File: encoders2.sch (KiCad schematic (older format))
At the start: 29 parts, among them U7 74HCT595, U9 74HC165

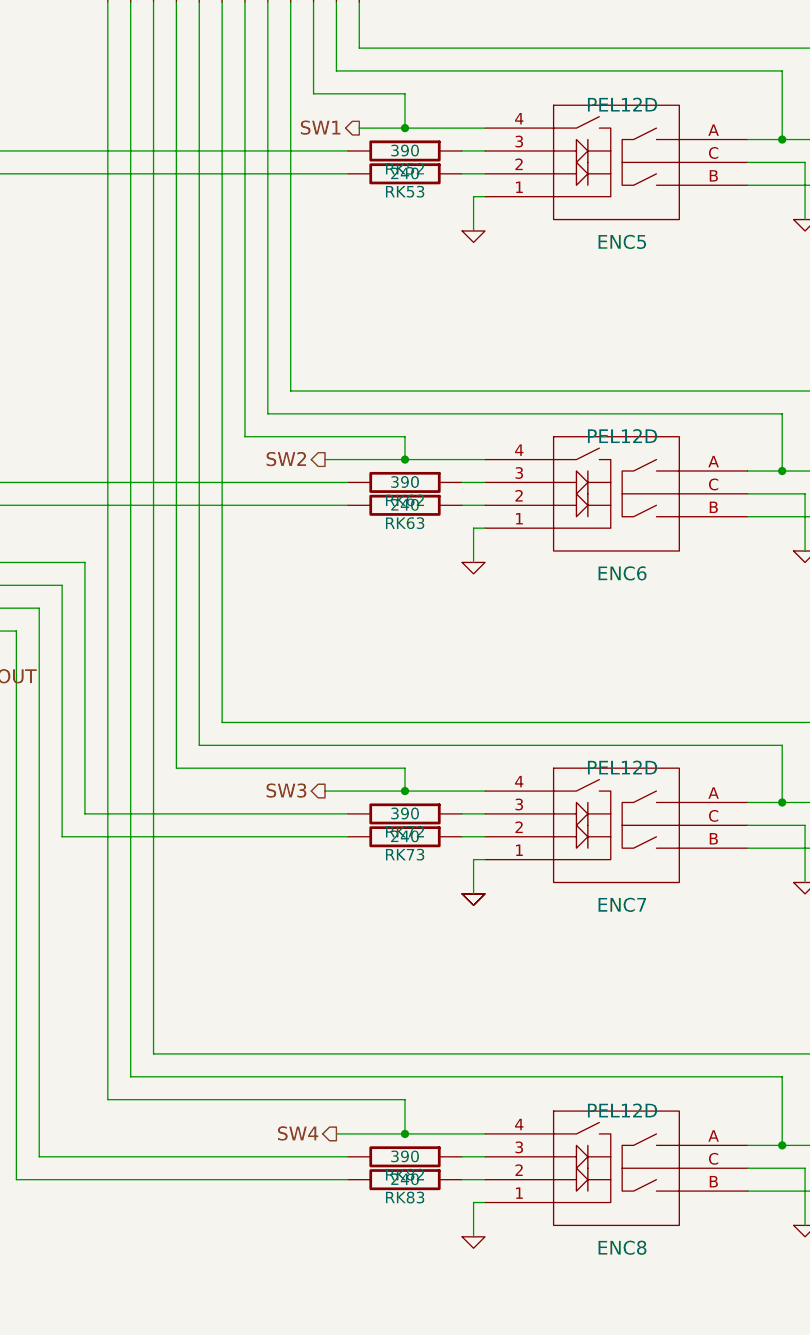
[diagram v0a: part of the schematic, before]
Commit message: Finished board CAD?
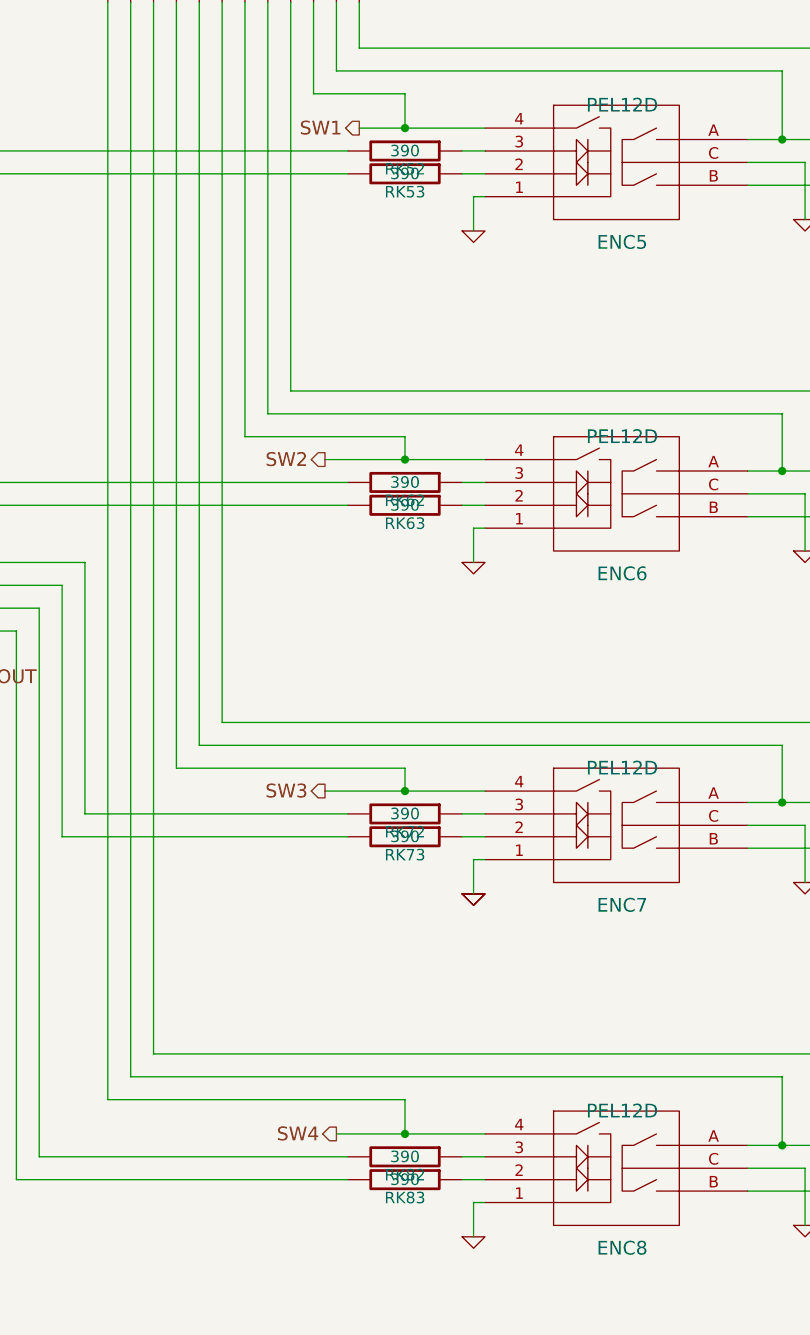
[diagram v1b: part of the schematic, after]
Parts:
- RK53, RK63, RK73, RK83: value 240 -> 390
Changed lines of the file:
@@
-EESchema Schematic File Version 2  date Sat 01 Jun 2013 11:43:44 AM CEST
+EESchema Schematic File Version 2  date Sat 08 Jun 2013 11:15:40 AM CEST
 LIBS:power
 LIBS:device
@@
 Sheet 8 10
 Title ""
-Date "1 jun 2013"
+Date "8 jun 2013"
 Rev ""
 Comp ""
@@
 $EndComp
 $Comp
-L +5V #PWR85
+L +5V #PWR090
 U 1 1 4F92B274
 P 1050 3200
-F 0 "#PWR85" H 1050 3290 20  0001 C CNN
+F 0 "#PWR090" H 1050 3290 20  0001 C CNN
 F 1 "+5V" H 1050 3290 30  0000 C CNN
 	1    1050 3200
@@
 NXP 74HCT595 will source up to 8mA to each output\nand seems to be 5V/3V compatible.
 $Comp
-L +3.3V #PWR100
+L +3.3V #PWR091
 U 1 1 4F92B272
 P 10300 5550
-F 0 "#PWR100" H 10300 5510 30  0001 C CNN
+F 0 "#PWR091" H 10300 5510 30  0001 C CNN
 F 1 "+3.3V" H 10300 5660 30  0000 C CNN
 	1    10300 5550
@@
 $EndComp
 $Comp
-L GND #PWR101
+L GND #PWR092
 U 1 1 4F92B234
 P 10300 6250
-F 0 "#PWR101" H 10300 6250 30  0001 C CNN
+F 0 "#PWR092" H 10300 6250 30  0001 C CNN
 F 1 "GND" H 10300 6180 30  0001 C CNN
 	1    10300 6250
@@
 $EndComp
 $Comp
-L GND #PWR88
+L GND #PWR093
 U 1 1 4F92B232
 P 1850 7150
-F 0 "#PWR88" H 1850 7150 30  0001 C CNN
+F 0 "#PWR093" H 1850 7150 30  0001 C CNN
 F 1 "GND" H 1850 7080 30  0001 C CNN
 	1    1850 7150
@@
 $EndComp
 $Comp
-L +5V #PWR87
+L +5V #PWR094
 U 1 1 4F829EA0
 P 1850 6500
-F 0 "#PWR87" H 1850 6590 20  0001 C CNN
+F 0 "#PWR094" H 1850 6590 20  0001 C CNN
 F 1 "+5V" H 1850 6590 30  0000 C CNN
 	1    1850 6500
@@
 $EndComp
 $Comp
-L +3.3V #PWR98
+L +3.3V #PWR095
 U 1 1 4F905A6B
 P 9450 3500
-F 0 "#PWR98" H 9450 3460 30  0001 C CNN
+F 0 "#PWR095" H 9450 3460 30  0001 C CNN
 F 1 "+3.3V" H 9450 3610 30  0000 C CNN
 	1    9450 3500
@@
 $EndComp
 $Comp
-L GND #PWR99
+L GND #PWR096
 U 1 1 4F905A6A
 P 9450 5250
-F 0 "#PWR99" H 9450 5250 30  0001 C CNN
+F 0 "#PWR096" H 9450 5250 30  0001 C CNN
 F 1 "GND" H 9450 5180 30  0001 C CNN
 	1    9450 5250
@@
 Needs to be 5V/3V compatible --> use HCT
 $Comp
-L GND #PWR86
+L GND #PWR097
 U 1 1 4F803213
 P 1050 4700
-F 0 "#PWR86" H 1050 4700 30  0001 C CNN
+F 0 "#PWR097" H 1050 4700 30  0001 C CNN
 F 1 "GND" H 1050 4630 30  0001 C CNN
 	1    1050 4700
@@
 $EndComp
 $Comp
-L GND #PWR91
+L GND #PWR098
 U 1 1 4F803206
 P 5150 5350
-F 0 "#PWR91" H 5150 5350 30  0001 C CNN
+F 0 "#PWR098" H 5150 5350 30  0001 C CNN
 F 1 "GND" H 5150 5280 30  0001 C CNN
 	1    5150 5350
@@
 $EndComp
 $Comp
-L GND #PWR89
+L GND #PWR099
 U 1 1 4F905A65
 P 5150 2450
-F 0 "#PWR89" H 5150 2450 30  0001 C CNN
+F 0 "#PWR099" H 5150 2450 30  0001 C CNN
 F 1 "GND" H 5150 2380 30  0001 C CNN
 	1    5150 2450
@@
 P 4850 2200
 F 0 "RK53" V 4930 2200 50  0000 C CNN
-F 1 "240" V 4850 2200 50  0000 C CNN
+F 1 "390" V 4850 2200 50  0000 C CNN
 	1    4850 2200
 	0    1    1    0
 $EndComp
 $Comp
-L GND #PWR94
+L GND #PWR0100
 U 1 1 4F92B25D
 P 6600 2400
-F 0 "#PWR94" H 6600 2400 30  0001 C CNN
+F 0 "#PWR0100" H 6600 2400 30  0001 C CNN
 F 1 "GND" H 6600 2330 30  0001 C CNN
 	1    6600 2400
@@
 $EndComp
 $Comp
-L GND #PWR95
+L GND #PWR0101
 U 1 1 4F92B250
 P 6600 3850
-F 0 "#PWR95" H 6600 3850 30  0001 C CNN
+F 0 "#PWR0101" H 6600 3850 30  0001 C CNN
 F 1 "GND" H 6600 3780 30  0001 C CNN
 	1    6600 3850
@@
 P 4850 3650
 F 0 "RK63" V 4930 3650 50  0000 C CNN
-F 1 "240" V 4850 3650 50  0000 C CNN
+F 1 "390" V 4850 3650 50  0000 C CNN
 	1    4850 3650
 	0    1    1    0
@@
 $EndComp
 $Comp
-L GND #PWR90
+L GND #PWR0102
 U 1 1 4F92B249
 P 5150 3900
-F 0 "#PWR90" H 5150 3900 30  0001 C CNN
+F 0 "#PWR0102" H 5150 3900 30  0001 C CNN
 F 1 "GND" H 5150 3830 30  0001 C CNN
 	1    5150 3900
@@
 $EndComp
 $Comp
-L GND #PWR92
+L GND #PWR0103
 U 1 1 4F92B245
 P 5150 5350
-F 0 "#PWR92" H 5150 5350 30  0001 C CNN
+F 0 "#PWR0103" H 5150 5350 30  0001 C CNN
 F 1 "GND" H 5150 5280 30  0001 C CNN
 	1    5150 5350
@@
 P 4850 5100
 F 0 "RK73" V 4930 5100 50  0000 C CNN
-F 1 "240" V 4850 5100 50  0000 C CNN
+F 1 "390" V 4850 5100 50  0000 C CNN
 	1    4850 5100
 	0    1    1    0
 $EndComp
 $Comp
-L GND #PWR96
+L GND #PWR0104
 U 1 1 4F92B207
 P 6600 5300
-F 0 "#PWR96" H 6600 5300 30  0001 C CNN
+F 0 "#PWR0104" H 6600 5300 30  0001 C CNN
 F 1 "GND" H 6600 5230 30  0001 C CNN
 	1    6600 5300
@@
 $EndComp
 $Comp
-L GND #PWR97
+L GND #PWR0105
 U 1 1 4F92B237
 P 6600 6800
-F 0 "#PWR97" H 6600 6800 30  0001 C CNN
+F 0 "#PWR0105" H 6600 6800 30  0001 C CNN
 F 1 "GND" H 6600 6730 30  0001 C CNN
 	1    6600 6800
@@
 P 4850 6600
 F 0 "RK83" V 4930 6600 50  0000 C CNN
-F 1 "240" V 4850 6600 50  0000 C CNN
+F 1 "390" V 4850 6600 50  0000 C CNN
 	1    4850 6600
 	0    1    1    0
@@
 $EndComp
 $Comp
-L GND #PWR93
+L GND #PWR0106
 U 1 1 4F92B1FA
 P 5150 6850
-F 0 "#PWR93" H 5150 6850 30  0001 C CNN
+F 0 "#PWR0106" H 5150 6850 30  0001 C CNN
 F 1 "GND" H 5150 6780 30  0001 C CNN
 	1    5150 6850
